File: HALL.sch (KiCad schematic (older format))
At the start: 8 parts, among them P6 CON_HALL

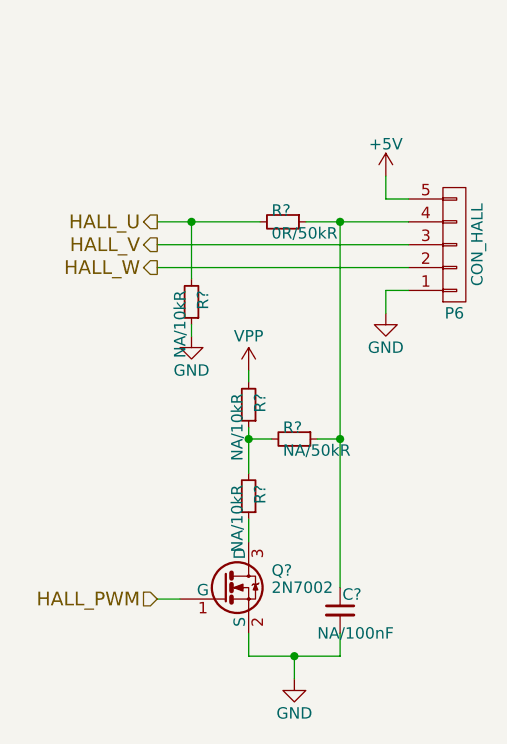
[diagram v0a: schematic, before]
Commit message: routed... at least for now
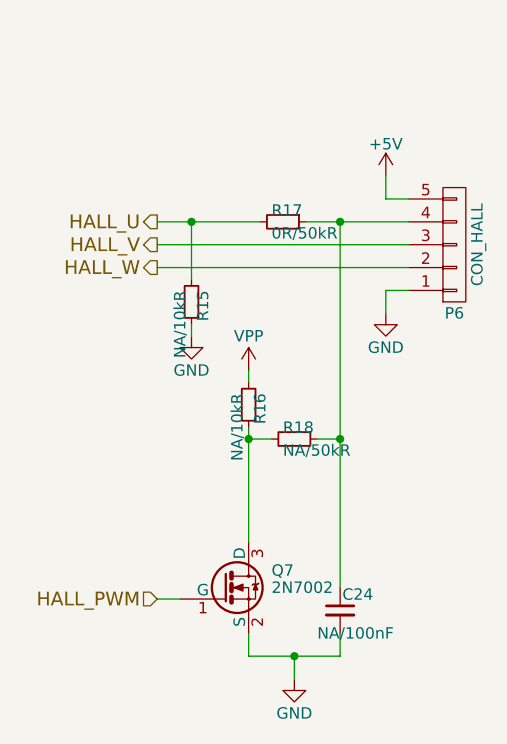
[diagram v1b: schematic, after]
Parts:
- removed R?: NA/10kR, symbol R_Small
- C24: renamed from C?; footprint (none) -> Capacitors_SMD:C_0603
- R15, R16, R17, R18: renamed from R?; footprint (none) -> Resistors_SMD:R_0603
- gave numbers to parts that had none: 1
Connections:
- net at Q7.3 (D): now also R16.1, R18.2
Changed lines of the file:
@@
 	2000 1500 2100 1500
 $Comp
-L GND #PWR049
+L GND #PWR052
 U 1 1 57ADAB3C
 P 2000 2000
-F 0 "#PWR049" H 2000 1750 50  0001 C CNN
+F 0 "#PWR052" H 2000 1750 50  0001 C CNN
 F 1 "GND" H 2000 1850 50  0000 C CNN
 F 2 "" H 2000 2000 50  0000 C CNN
@@
 HALL_W
 $Comp
-L +5V #PWR?
+L +5V #PWR053
 U 1 1 580F5FAC
 P 2000 1400
-F 0 "#PWR?" H 2000 1250 50  0001 C CNN
+F 0 "#PWR053" H 2000 1250 50  0001 C CNN
 F 1 "+5V" H 2000 1540 50  0000 C CNN
 F 2 "" H 2000 1400 50  0000 C CNN
@@
 $EndComp
 $Comp
-L C_Small C?
+L C_Small C24
 U 1 1 580F6E53
 P 1800 3300
-F 0 "C?" H 1810 3370 50  0000 L CNN
+F 0 "C24" H 1810 3370 50  0000 L CNN
 F 1 "NA/100nF" H 1700 3200 50  0000 L CNN
-F 2 "" H 1800 3300 50  0000 C CNN
+F 2 "Capacitors_SMD:C_0603" H 1800 3300 50  0001 C CNN
 F 3 "" H 1800 3300 50  0000 C CNN
 	1    1800 3300
@@
 $EndComp
 $Comp
-L GND #PWR?
+L GND #PWR054
 U 1 1 580F6E9B
 P 1600 3600
-F 0 "#PWR?" H 1600 3350 50  0001 C CNN
+F 0 "#PWR054" H 1600 3350 50  0001 C CNN
 F 1 "GND" H 1600 3450 50  0000 C CNN
 F 2 "" H 1600 3600 50  0000 C CNN
@@
 $EndComp
 $Comp
-L R_Small R?
+L R_Small R18
 U 1 1 580F71C7
 P 1600 2550
-F 0 "R?" V 1550 2500 50  0000 L CNN
+F 0 "R18" V 1550 2500 50  0000 L CNN
 F 1 "NA/50kR" V 1650 2500 50  0000 L CNN
-F 2 "" H 1600 2550 50  0000 C CNN
+F 2 "Resistors_SMD:R_0603" H 1600 2550 50  0001 C CNN
 F 3 "" H 1600 2550 50  0000 C CNN
 	1    1600 2550
@@
 	1000 1800 2100 1800
 $Comp
-L R_Small R?
+L R_Small R17
 U 1 1 580F173E
 P 1550 1600
-F 0 "R?" V 1500 1550 50  0000 L CNN
+F 0 "R17" V 1500 1550 50  0000 L CNN
 F 1 "0R/50kR" V 1600 1550 50  0000 L CNN
-F 2 "" H 1550 1600 50  0000 C CNN
+F 2 "Resistors_SMD:R_0603" H 1550 1600 50  0001 C CNN
 F 3 "" H 1550 1600 50  0000 C CNN
 	1    1550 1600
@@
 	1000 1600 1450 1600
 $Comp
-L R_Small R?
+L R_Small R15
 U 1 1 580F1844
 P 1150 1950
-F 0 "R?" V 1100 1900 50  0000 L CNN
+F 0 "R15" V 1100 1900 50  0000 L CNN
 F 1 "NA/10kR" V 1200 1900 50  0000 L CNN
-F 2 "" H 1150 1950 50  0000 C CNN
+F 2 "Resistors_SMD:R_0603" H 1150 1950 50  0001 C CNN
 F 3 "" H 1150 1950 50  0000 C CNN
 	1    1150 1950
@@
 Connection ~ 1150 1600
 $Comp
-L VPP #PWR?
+L VPP #PWR055
 U 1 1 580F18F3
 P 1400 2250
-F 0 "#PWR?" H 1400 2100 50  0001 C CNN
+F 0 "#PWR055" H 1400 2100 50  0001 C CNN
 F 1 "VPP" H 1400 2400 50  0000 C CNN
 F 2 "" H 1400 2250 50  0000 C CNN
@@
 $EndComp
 $Comp
-L 2N7002 Q?
+L 2N7002 Q7
 U 1 1 580F19BB
 P 1300 3200
-F 0 "Q?" H 1500 3275 50  0000 L CNN
+F 0 "Q7" H 1500 3275 50  0000 L CNN
 F 1 "2N7002" H 1500 3200 50  0000 L CNN
 F 2 "TO_SOT_Packages_SMD:SOT-23" H 1500 3125 50  0001 L CIN
@@
 Connection ~ 1600 3500
 $Comp
-L R_Small R?
+L R_Small R16
 U 1 1 580F1ACA
 P 1400 2400
-F 0 "R?" V 1350 2350 50  0000 L CNN
+F 0 "R16" V 1350 2350 50  0000 L CNN
 F 1 "NA/10kR" V 1450 2350 50  0000 L CNN
-F 2 "" H 1400 2400 50  0000 C CNN
+F 2 "Resistors_SMD:R_0603" H 1400 2400 50  0001 C CNN
 F 3 "" H 1400 2400 50  0000 C CNN
 	1    1400 2400
@@
 	1500 2550 1400 2550
 Wire Wire Line
-	1400 2500 1400 2700
+	1400 2500 1400 3000
 Connection ~ 1400 2550
 Wire Wire Line
 	1000 3250 1100 3250
 $Comp
-L GND #PWR?
+L GND #PWR056
 U 1 1 580F1E73
 P 1150 2100
-F 0 "#PWR?" H 1150 1850 50  0001 C CNN
+F 0 "#PWR056" H 1150 1850 50  0001 C CNN
 F 1 "GND" H 1150 1950 50  0000 C CNN
 F 2 "" H 1150 2100 50  0000 C CNN
@@
 Wire Wire Line
 	1150 2100 1150 2050
-$Comp
-L R_Small R?
-U 1 1 580F218F
-P 1400 2800
-F 0 "R?" V 1350 2750 50  0000 L CNN
-F 1 "NA/10kR" V 1450 2750 50  0000 L CNN
-F 2 "" H 1400 2800 50  0000 C CNN
-F 3 "" H 1400 2800 50  0000 C CNN
-	1    1400 2800
-	-1   0    0    1
-$EndComp
-Wire Wire Line
-	1400 2900 1400 3000
 $EndSCHEMATC

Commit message: long forgotten commit of something I did half a year ago -.-
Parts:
- removed C24: NA/100nF, Capacitors_SMD:C_0603, symbol C_Small
- removed Q7: 2N7002, TO_SOT_Packages_SMD:SOT-23, symbol 2N7002
- removed R15, R16: NA/10kR, Resistors_SMD:R_0603, symbol R_Small
- removed R17: 0R/50kR, Resistors_SMD:R_0603, symbol R_Small
- removed R18: NA/50kR, Resistors_SMD:R_0603, symbol R_Small
- added R16, R17, R18: 47kR, Resistor_SMD:R_0603_1608Metric, symbol bldc-controller-rescue:R_Small
- P6: footprint Terminal_Blocks:TerminalBlock_Pheonix_MPT-2.54mm_5pol -> Connector_PinHeader_2.54mm:PinHeader_1x05_P2.54mm_Horizontal; symbol CONN_01X05 -> bldc-controller-rescue:CONN_01X05
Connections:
- net labels removed: GND, HALL_PWM, VPP
- wire segments 20 -> 18
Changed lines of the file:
@@
-EESchema Schematic File Version 2
-LIBS:bldc-controller-rescue
-LIBS:power
-LIBS:device
-LIBS:transistors
-LIBS:conn
-LIBS:linear
-LIBS:regul
-LIBS:74xx
-LIBS:cmos4000
-LIBS:adc-dac
-LIBS:memory
-LIBS:xilinx
-LIBS:microcontrollers
-LIBS:dsp
-LIBS:microchip
-LIBS:analog_switches
-LIBS:motorola
-LIBS:texas
-LIBS:intel
-LIBS:audio
-LIBS:interface
-LIBS:digital-audio
-LIBS:philips
-LIBS:display
-LIBS:cypress
-LIBS:siliconi
-LIBS:opto
-LIBS:atmel
-LIBS:contrib
-LIBS:valves
-LIBS:Power_Management
-LIBS:st-microelectronics
-LIBS:stm32
-LIBS:w_analog
-LIBS:mpu6000
+EESchema Schematic File Version 4
 LIBS:bldc-controller-cache
-EELAYER 25 0
+EELAYER 29 0
 EELAYER END
 $Descr A4 11693 8268
@@
 $EndDescr
 $Comp
-L CONN_01X05 P6
+L bldc-controller-rescue:CONN_01X05 P6
 U 1 1 57ADAAC3
 P 2300 1700
 F 0 "P6" H 2300 2000 50  0000 C CNN
 F 1 "CON_HALL" V 2400 1700 50  0000 C CNN
-F 2 "Terminal_Blocks:TerminalBlock_Pheonix_MPT-2.54mm_5pol" H 2300 1700 50  0001 C CNN
+F 2 "Connector_PinHeader_2.54mm:PinHeader_1x05_P2.54mm_Horizontal" H 2300 1700 50  0001 C CNN
 F 3 "" H 2300 1700 50  0000 C CNN
 	1    2300 1700
-	1    0    0    1
+	1    0    0    -1
 $EndComp
 Wire Wire Line
@@
 Wire Wire Line
 	2000 1500 2100 1500
-$Comp
-L GND #PWR052
-U 1 1 57ADAB3C
-P 2000 2000
-F 0 "#PWR052" H 2000 1750 50  0001 C CNN
-F 1 "GND" H 2000 1850 50  0000 C CNN
-F 2 "" H 2000 2000 50  0000 C CNN
-F 3 "" H 2000 2000 50  0000 C CNN
-	1    2000 2000
-	1    0    0    -1
-$EndComp
-Wire Wire Line
-	2000 2000 2000 1900
 Wire Wire Line
 	2000 1900 2100 1900
@@
 HALL_W
 $Comp
-L +5V #PWR053
+L bldc-controller-rescue:+5V #PWR053
 U 1 1 580F5FAC
 P 2000 1400
+AR Path="/580F5FAC" Ref="#PWR053"  Part="1"
+AR Path="/580FABC4/580F5FAC" Ref="#PWR053"  Part="1"
 F 0 "#PWR053" H 2000 1250 50  0001 C CNN
 F 1 "+5V" H 2000 1540 50  0000 C CNN
@@
 	1    0    0    -1
 $EndComp
+Wire Wire Line
+	1000 1700 1550 1700
+Wire Wire Line
+	1000 1800 1700 1800
 $Comp
-L C_Small C24
-U 1 1 580F6E53
-P 1800 3300
-F 0 "C24" H 1810 3370 50  0000 L CNN
-F 1 "NA/100nF" H 1700 3200 50  0000 L CNN
-F 2 "Capacitors_SMD:C_0603" H 1800 3300 50  0001 C CNN
-F 3 "" H 1800 3300 50  0000 C CNN
-	1    1800 3300
-	1    0    0    -1
+L bldc-controller-rescue:R_Small R16
+U 1 1 5D30EF33
+P 1400 1250
+F 0 "R16" V 1350 1200 50  0000 L CNN
+F 1 "47kR" V 1450 1200 50  0000 L CNN
+F 2 "Resistor_SMD:R_0603_1608Metric" H 1400 1250 50  0001 C CNN
+F 3 "" H 1400 1250 50  0000 C CNN
+	1    1400 1250
+	-1   0    0    1
 $EndComp
 $Comp
-L GND #PWR054
-U 1 1 580F6E9B
-P 1600 3600
-F 0 "#PWR054" H 1600 3350 50  0001 C CNN
-F 1 "GND" H 1600 3450 50  0000 C CNN
-F 2 "" H 1600 3600 50  0000 C CNN
-F 3 "" H 1600 3600 50  0000 C CNN
-	1    1600 3600
-	1    0    0    -1
+L bldc-controller-rescue:R_Small R17
+U 1 1 5D30F3A9
+P 1550 1250
+F 0 "R17" V 1500 1200 50  0000 L CNN
+F 1 "47kR" V 1600 1200 50  0000 L CNN
+F 2 "Resistor_SMD:R_0603_1608Metric" H 1550 1250 50  0001 C CNN
+F 3 "" H 1550 1250 50  0000 C CNN
+	1    1550 1250
+	-1   0    0    1
 $EndComp
 $Comp
-L R_Small R18
-U 1 1 580F71C7
-P 1600 2550
-F 0 "R18" V 1550 2500 50  0000 L CNN
-F 1 "NA/50kR" V 1650 2500 50  0000 L CNN
-F 2 "Resistors_SMD:R_0603" H 1600 2550 50  0001 C CNN
-F 3 "" H 1600 2550 50  0000 C CNN
-	1    1600 2550
-	0    1    1    0
-$EndComp
-Wire Wire Line
-	1650 1600 2100 1600
-Wire Wire Line
-	1000 1700 2100 1700
-Text HLabel 1000 3250 0    60   Input ~ 0
-HALL_PWM
-Wire Wire Line
-	1700 2550 1800 2550
-Wire Wire Line
-	1800 1600 1800 3200
-Connection ~ 1800 1600
-Connection ~ 1800 2550
-Wire Wire Line
-	1000 1800 2100 1800
-$Comp
-L R_Small R17
-U 1 1 580F173E
-P 1550 1600
-F 0 "R17" V 1500 1550 50  0000 L CNN
-F 1 "0R/50kR" V 1600 1550 50  0000 L CNN
-F 2 "Resistors_SMD:R_0603" H 1550 1600 50  0001 C CNN
-F 3 "" H 1550 1600 50  0000 C CNN
-	1    1550 1600
-	0    1    1    0
-$EndComp
-Wire Wire Line
-	1000 1600 1450 1600
-$Comp
-L R_Small R15
-U 1 1 580F1844
-P 1150 1950
-F 0 "R15" V 1100 1900 50  0000 L CNN
-F 1 "NA/10kR" V 1200 1900 50  0000 L CNN
-F 2 "Resistors_SMD:R_0603" H 1150 1950 50  0001 C CNN
-F 3 "" H 1150 1950 50  0000 C CNN
-	1    1150 1950
+L bldc-controller-rescue:R_Small R18
+U 1 1 5D30F5F4
+P 1700 1250
+F 0 "R18" V 1650 1200 50  0000 L CNN
+F 1 "47kR" V 1750 1200 50  0000 L CNN
+F 2 "Resistor_SMD:R_0603_1608Metric" H 1700 1250 50  0001 C CNN
+F 3 "" H 1700 1250 50  0000 C CNN
+	1    1700 1250
 	-1   0    0    1
 $EndComp
 Wire Wire Line
-	1150 1850 1150 1600
-Connection ~ 1150 1600
+	1400 1350 1400 1600
+Connection ~ 1400 1600
+Wire Wire Line
+	1400 1600 2100 1600
+Wire Wire Line
+	1550 1350 1550 1700
+Connection ~ 1550 1700
+Wire Wire Line
+	1550 1700 2100 1700
+Wire Wire Line
+	1700 1350 1700 1800
+Connection ~ 1700 1800
+Wire Wire Line
+	1700 1800 2100 1800
 $Comp
-L VPP #PWR055
-U 1 1 580F18F3
-P 1400 2250
-F 0 "#PWR055" H 1400 2100 50  0001 C CNN
-F 1 "VPP" H 1400 2400 50  0000 C CNN
-F 2 "" H 1400 2250 50  0000 C CNN
-F 3 "" H 1400 2250 50  0000 C CNN
-	1    1400 2250
-	1    0    0    -1
-$EndComp
-$Comp
-L 2N7002 Q7
-U 1 1 580F19BB
-P 1300 3200
-F 0 "Q7" H 1500 3275 50  0000 L CNN
-F 1 "2N7002" H 1500 3200 50  0000 L CNN
-F 2 "TO_SOT_Packages_SMD:SOT-23" H 1500 3125 50  0001 L CIN
-F 3 "" H 1300 3200 50  0000 L CNN
-	1    1300 3200
+L bldc-controller-rescue:+5V #PWR?
+U 1 1 5D30FE82
+P 1550 900
+AR Path="/5D30FE82" Ref="#PWR?"  Part="1"
+AR Path="/580FABC4/5D30FE82" Ref="#PWR0101"  Part="1"
+F 0 "#PWR0101" H 1550 750 50  0001 C CNN
+F 1 "+5V" H 1550 1040 50  0000 C CNN
+F 2 "" H 1550 900 50  0000 C CNN
+F 3 "" H 1550 900 50  0000 C CNN
+	1    1550 900
 	1    0    0    -1
 $EndComp
 Wire Wire Line
-	1400 3400 1400 3500
+	1550 900  1550 1000
 Wire Wire Line
-	1400 3500 1800 3500
+	1400 1150 1400 1000
 Wire Wire Line
-	1800 3500 1800 3400
+	1400 1000 1550 1000
+Connection ~ 1550 1000
 Wire Wire Line
-	1600 3600 1600 3500
-Connection ~ 1600 3500
-$Comp
-L R_Small R16
-U 1 1 580F1ACA
-P 1400 2400
-F 0 "R16" V 1350 2350 50  0000 L CNN
-F 1 "NA/10kR" V 1450 2350 50  0000 L CNN
-F 2 "Resistors_SMD:R_0603" H 1400 2400 50  0001 C CNN
-F 3 "" H 1400 2400 50  0000 C CNN
-	1    1400 2400
-	-1   0    0    1
-$EndComp
+	1550 1000 1550 1150
 Wire Wire Line
-	1400 2250 1400 2300
+	1700 1150 1700 1000
 Wire Wire Line
-	1500 2550 1400 2550
+	1700 1000 1550 1000
 Wire Wire Line
-	1400 2500 1400 3000
-Connection ~ 1400 2550
-Wire Wire Line
-	1000 3250 1100 3250
-$Comp
-L GND #PWR056
-U 1 1 580F1E73
-P 1150 2100
-F 0 "#PWR056" H 1150 1850 50  0001 C CNN
-F 1 "GND" H 1150 1950 50  0000 C CNN
-F 2 "" H 1150 2100 50  0000 C CNN
-F 3 "" H 1150 2100 50  0000 C CNN
-	1    1150 2100
-	1    0    0    -1
-$EndComp
-Wire Wire Line
-	1150 2100 1150 2050
+	1000 1600 1400 1600
 $EndSCHEMATC
